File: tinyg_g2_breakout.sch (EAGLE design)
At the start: 23 parts

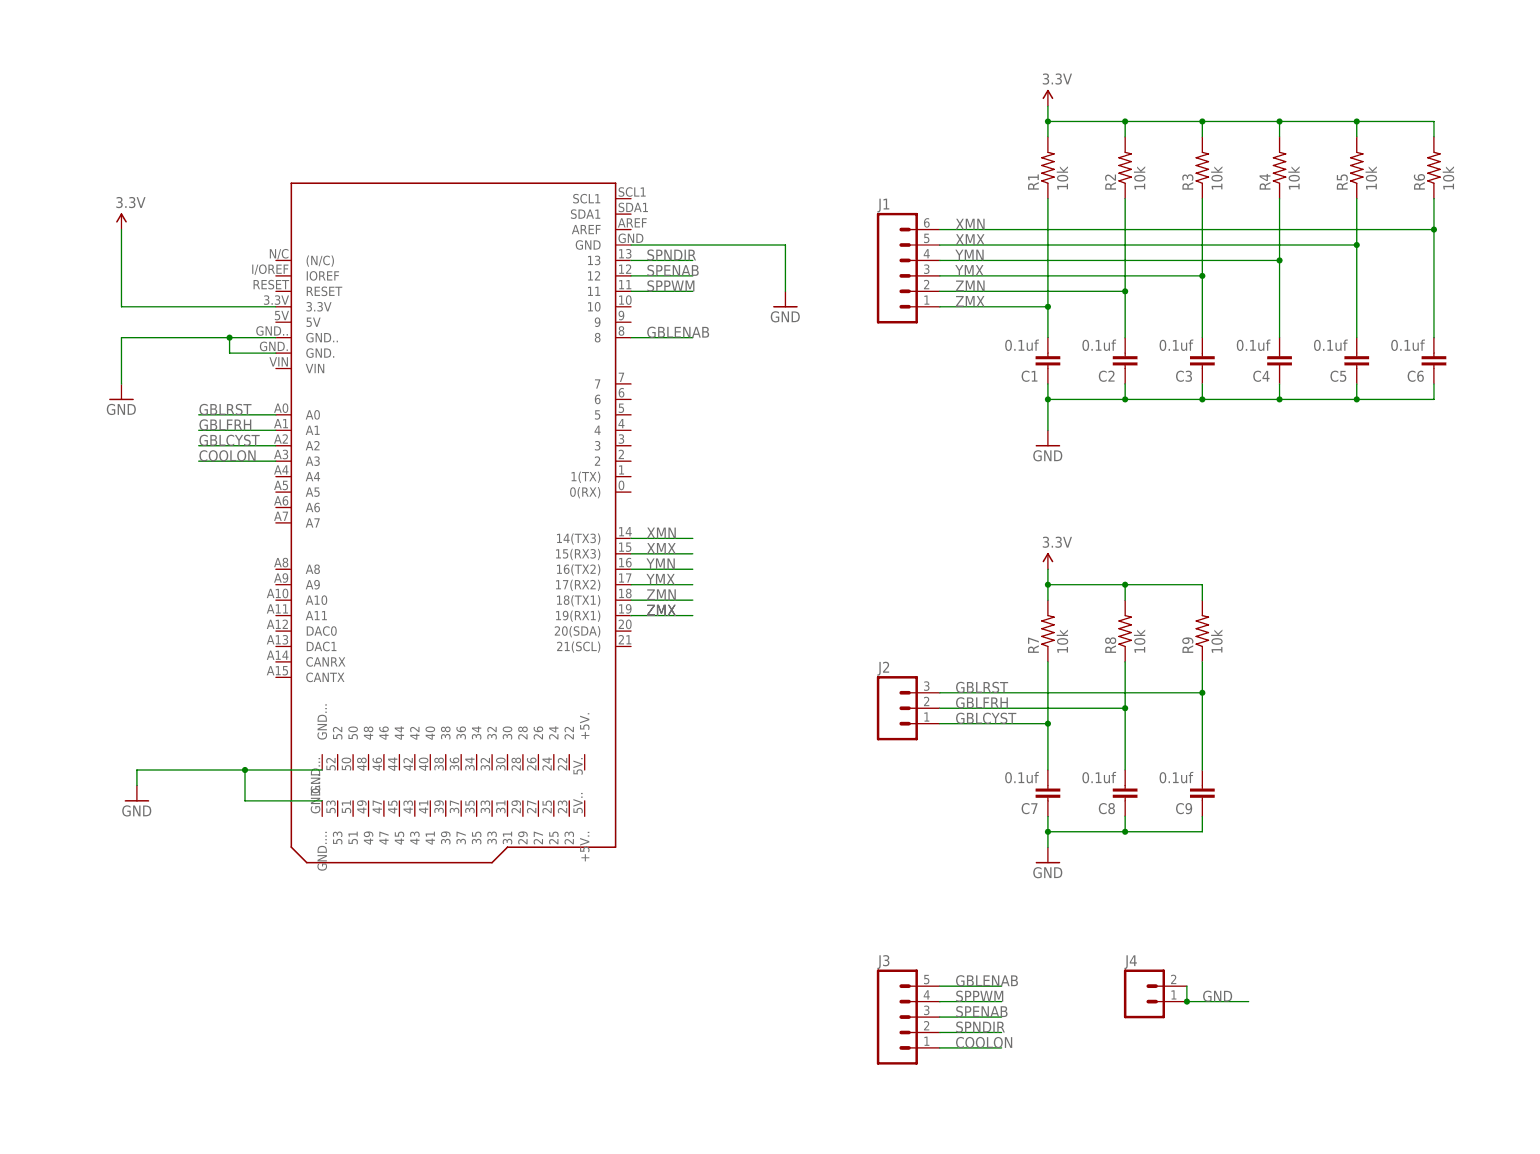
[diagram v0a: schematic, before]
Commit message: Updated files
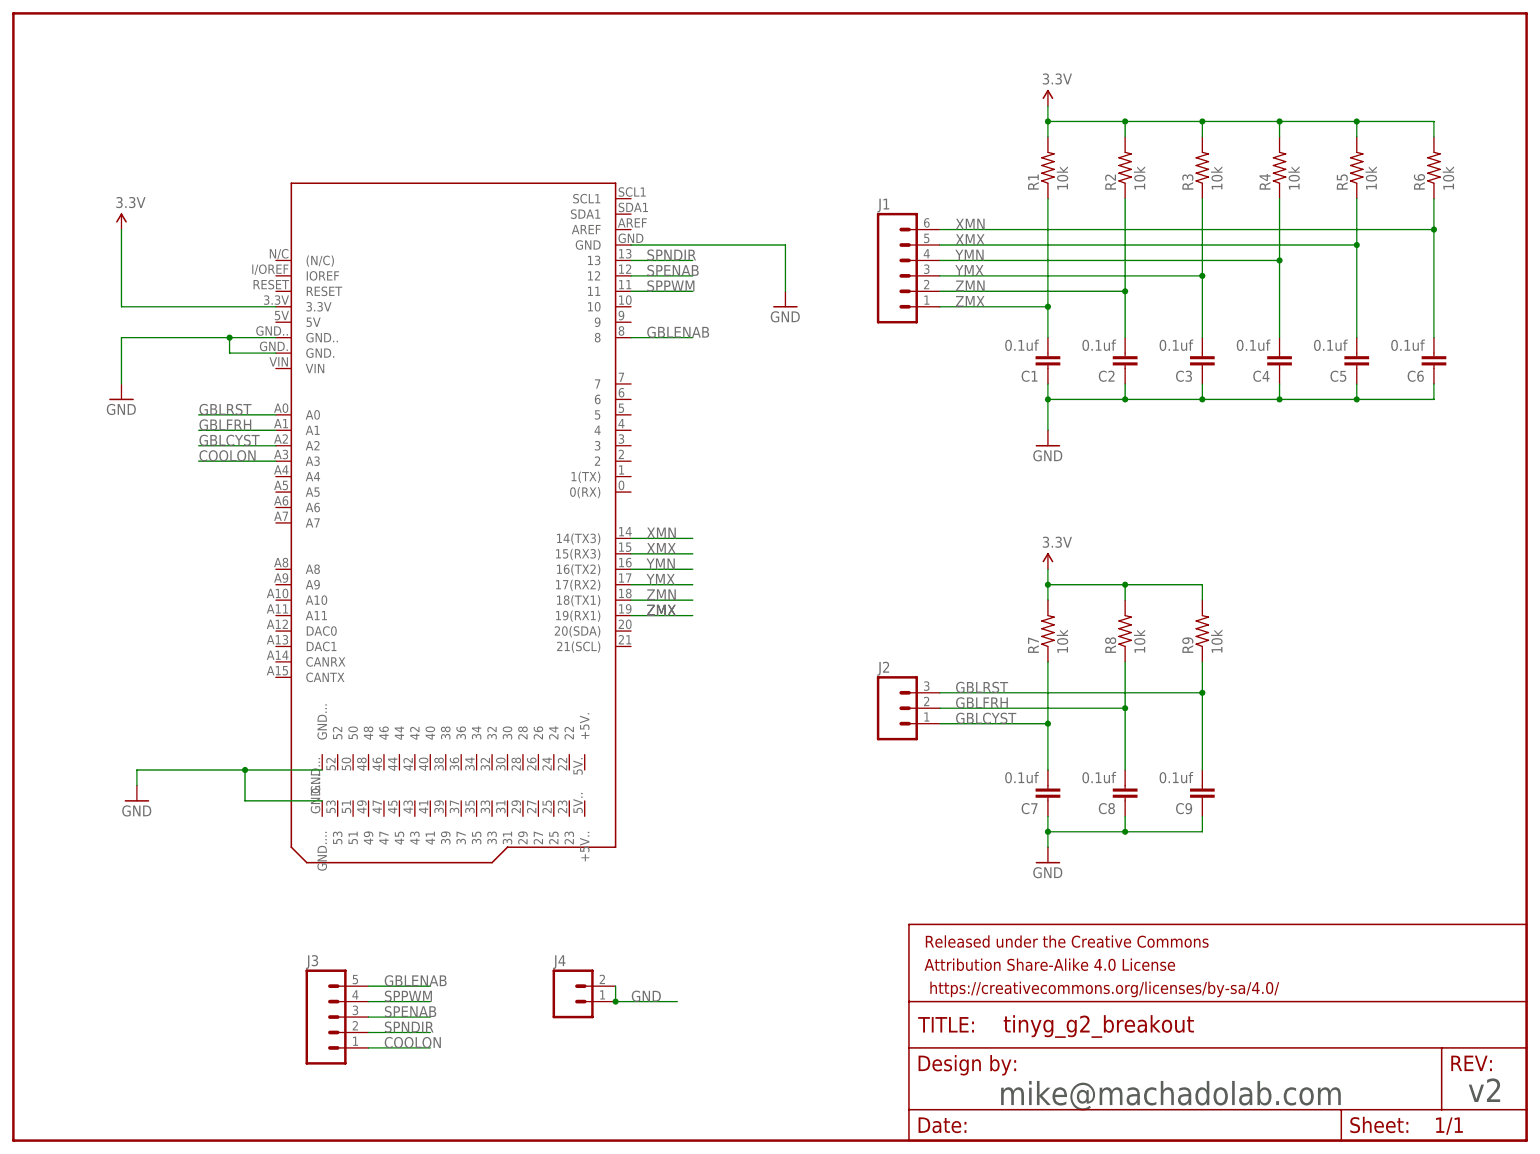
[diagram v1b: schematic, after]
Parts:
- added FRAME1: v1, SparkFun-Aesthetics:FRAME-LETTER
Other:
- note added: "mike@machadolab.com"
- note added: "v2"
- moved on the sheet: J3, J4
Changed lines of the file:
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@@
 <part name="GND5" library="SparkFun-Aesthetics" deviceset="GND" device=""/>
 <part name="SUPPLY3" library="SparkFun-Aesthetics" deviceset="3.3V" device=""/>
+<part name="FRAME1" library="SparkFun-Aesthetics" deviceset="FRAME-LETTER" device="" value="v1"/>
 </parts>
 <sheets>
 <sheet>
 <plain>
+<text x="165.608" y="-49.53" size="3.81" layer="97">v2</text>
+<text x="88.392" y="-50.038" size="3.81" layer="97">mike@machadolab.com</text>
 </plain>
 <instances>
 <instance part="PCB1" gate="G$1" x="0" y="55.88" rot="R270"/>
-<instance part="J4" gate="G$1" x="111.76" y="-33.02"/>
+<instance part="J4" gate="G$1" x="17.78" y="-33.02"/>
 <instance part="J1" gate="G$1" x="73.66" y="86.36"/>
 <instance part="R1" gate="G$1" x="96.52" y="104.14" rot="R90"/>
@@
 <instance part="GND2" gate="1" x="96.52" y="-10.16"/>
 <instance part="J2" gate="J$1" x="71.12" y="15.24"/>
-<instance part="J3" gate="G$1" x="71.12" y="-35.56"/>
+<instance part="J3" gate="G$1" x="-22.86" y="-35.56"/>
 <instance part="GND3" gate="1" x="-55.88" y="66.04"/>
 <instance part="GND4" gate="1" x="53.34" y="81.28"/>
 <instance part="GND5" gate="1" x="-53.34" y="0"/>
 <instance part="SUPPLY3" gate="G$1" x="-55.88" y="93.98"/>
+<instance part="FRAME1" gate="G$1" x="-73.66" y="-55.88"/>
+<instance part="FRAME1" gate="V" x="73.66" y="-55.88"/>
 </instances>
 <busses>
@@
 </segment>
 <segment>
-<wire x1="78.74" y1="-30.48" x2="88.9" y2="-30.48" width="0.1524" layer="91"/>
-<label x="81.28" y="-30.48" size="1.778" layer="95"/>
+<wire x1="-15.24" y1="-30.48" x2="-5.08" y2="-30.48" width="0.1524" layer="91"/>
+<label x="-12.7" y="-30.48" size="1.778" layer="95"/>
 <pinref part="J3" gate="G$1" pin="5"/>
 </segment>
@@
 </segment>
 <segment>
-<wire x1="78.74" y1="-33.02" x2="88.9" y2="-33.02" width="0.1524" layer="91"/>
-<label x="81.28" y="-33.02" size="1.778" layer="95"/>
+<wire x1="-15.24" y1="-33.02" x2="-5.08" y2="-33.02" width="0.1524" layer="91"/>
+<label x="-12.7" y="-33.02" size="1.778" layer="95"/>
 <pinref part="J3" gate="G$1" pin="4"/>
 </segment>
@@
 <segment>
 <pinref part="J3" gate="G$1" pin="1"/>
-<wire x1="78.74" y1="-40.64" x2="88.9" y2="-40.64" width="0.1524" layer="91"/>
-<label x="81.28" y="-40.64" size="1.778" layer="95"/>
+<wire x1="-15.24" y1="-40.64" x2="-5.08" y2="-40.64" width="0.1524" layer="91"/>
+<label x="-12.7" y="-40.64" size="1.778" layer="95"/>
 </segment>
 </net>
@@
 <pinref part="J4" gate="G$1" pin="2"/>
 <pinref part="J4" gate="G$1" pin="1"/>
-<wire x1="119.38" y1="-30.48" x2="119.38" y2="-33.02" width="0.1524" layer="91"/>
-<wire x1="119.38" y1="-33.02" x2="129.54" y2="-33.02" width="0.1524" layer="91"/>
-<junction x="119.38" y="-33.02"/>
-<label x="121.92" y="-33.02" size="1.778" layer="95"/>
+<wire x1="25.4" y1="-30.48" x2="25.4" y2="-33.02" width="0.1524" layer="91"/>
+<wire x1="25.4" y1="-33.02" x2="35.56" y2="-33.02" width="0.1524" layer="91"/>
+<junction x="25.4" y="-33.02"/>
+<label x="27.94" y="-33.02" size="1.778" layer="95"/>
 </segment>
 <segment>
@@
 </segment>
 <segment>
-<wire x1="78.74" y1="-35.56" x2="88.9" y2="-35.56" width="0.1524" layer="91"/>
-<label x="81.28" y="-35.56" size="1.778" layer="95"/>
+<wire x1="-15.24" y1="-35.56" x2="-5.08" y2="-35.56" width="0.1524" layer="91"/>
+<label x="-12.7" y="-35.56" size="1.778" layer="95"/>
 <pinref part="J3" gate="G$1" pin="3"/>
 </segment>
@@
 </segment>
 <segment>
-<wire x1="78.74" y1="-38.1" x2="88.9" y2="-38.1" width="0.1524" layer="91"/>
-<label x="81.28" y="-38.1" size="1.778" layer="95"/>
+<wire x1="-15.24" y1="-38.1" x2="-5.08" y2="-38.1" width="0.1524" layer="91"/>
+<label x="-12.7" y="-38.1" size="1.778" layer="95"/>
 <pinref part="J3" gate="G$1" pin="2"/>
 </segment>
